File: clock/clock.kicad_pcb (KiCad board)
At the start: 2 copper layers, 100 x 50 mm, 165 parts, among them J1 Conn_02x05_Odd_Even, P1 Conn_WallPlug, U1 74HC596, U10 74HC596, U11 LPC804-TSSOP24, U2 74HC596, U3 74HC596, U4 74HC596, U5 74HC596, U6 74HC596, U7 L78L33ABU, U8 74HC596, U9 74HC596

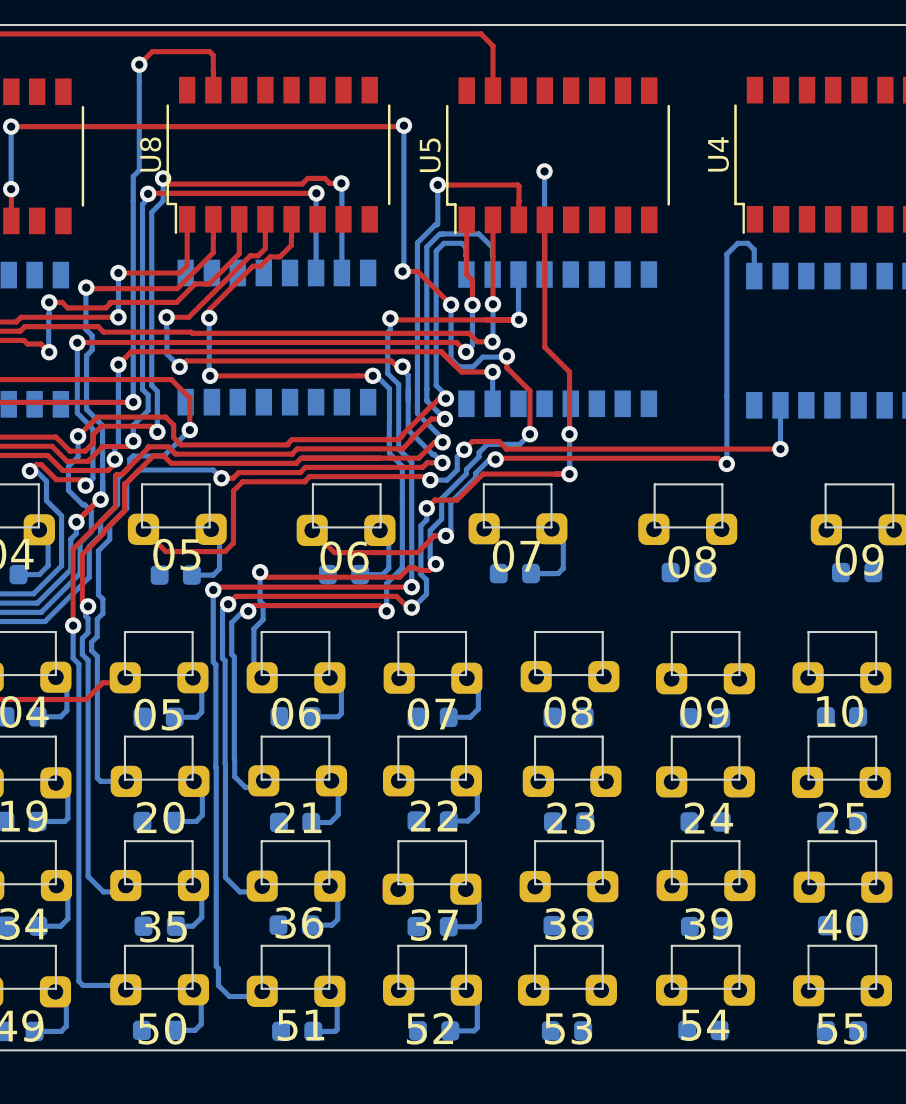
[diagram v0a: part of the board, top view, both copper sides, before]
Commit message: Saving routing progress. 50% done
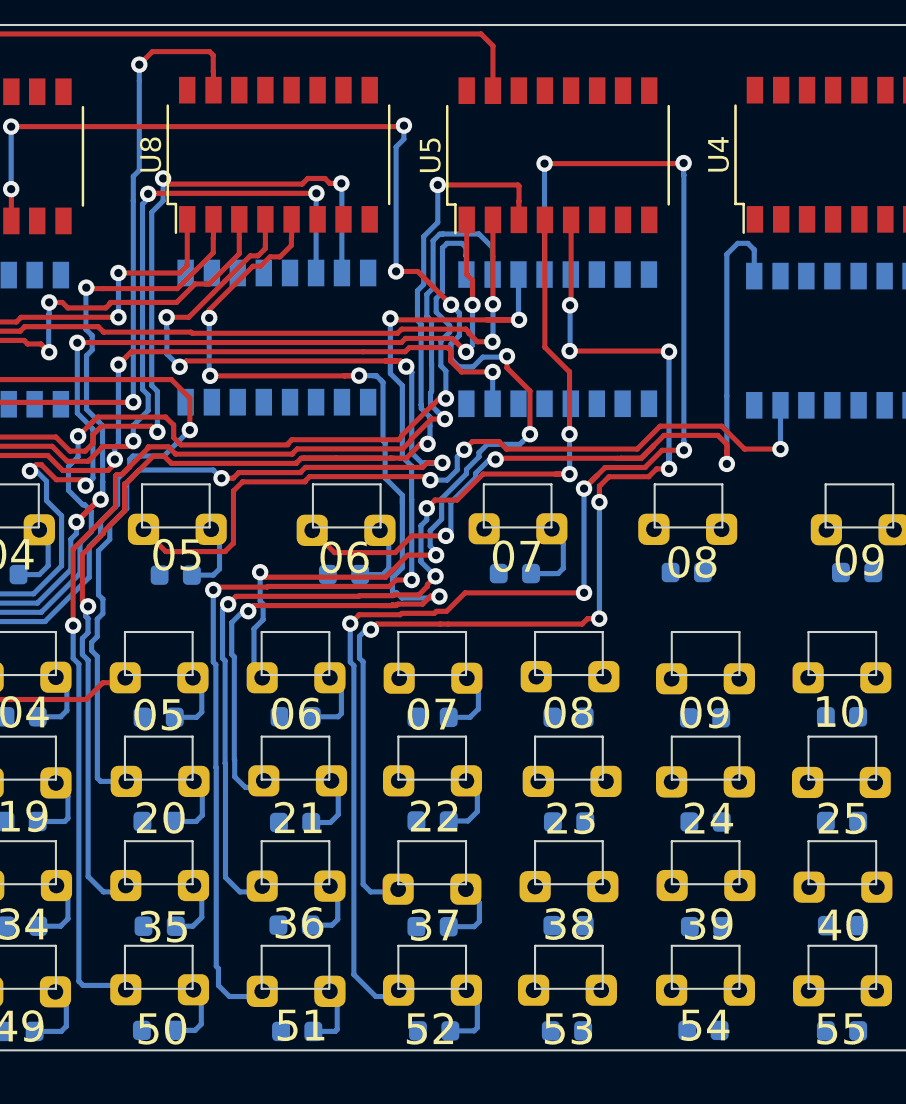
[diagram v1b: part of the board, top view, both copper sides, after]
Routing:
- net M52: track 5.03 -> 70.4 mm, vias 1 -> 6
- net M37: track 0.00 -> 53.7 mm, vias 0 -> 7
- net M21: track 47.5 -> 53.6 mm
- net H06: track 37.2 -> 40.7 mm
- net M20: track 60.5 -> 61.5 mm
- net H05: track 38.0 -> 38.9 mm
- net M35: track 64.2 -> 63.3 mm
- net M48: track 69.7 -> 69.1 mm
